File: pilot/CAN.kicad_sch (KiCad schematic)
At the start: 13 parts, among them IC1 TJA1050T, J4 Conn_01x02, U5 MCP2515-xSO, Y2 ABLS-8.000MHZ-12-B-4-Y-T

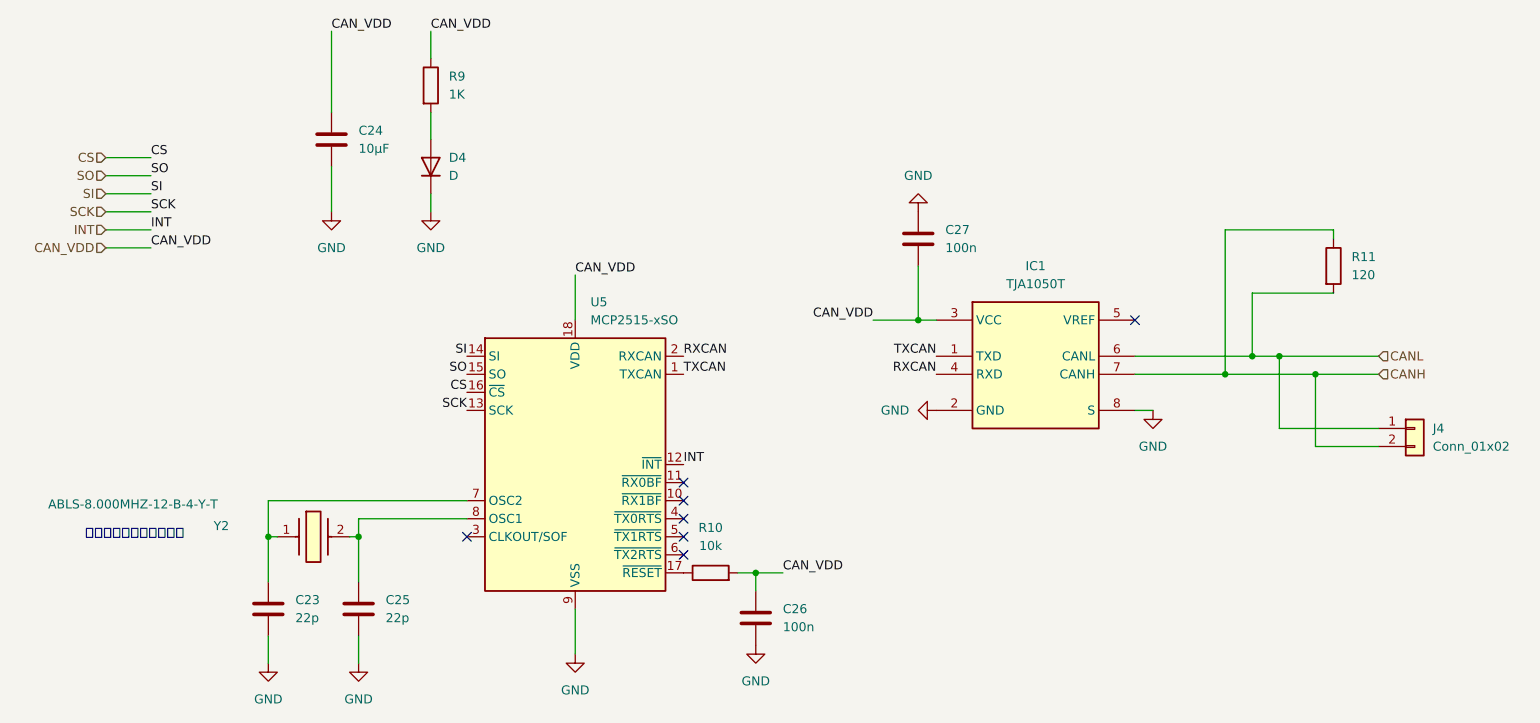
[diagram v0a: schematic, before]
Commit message: 2026/02/12/1628
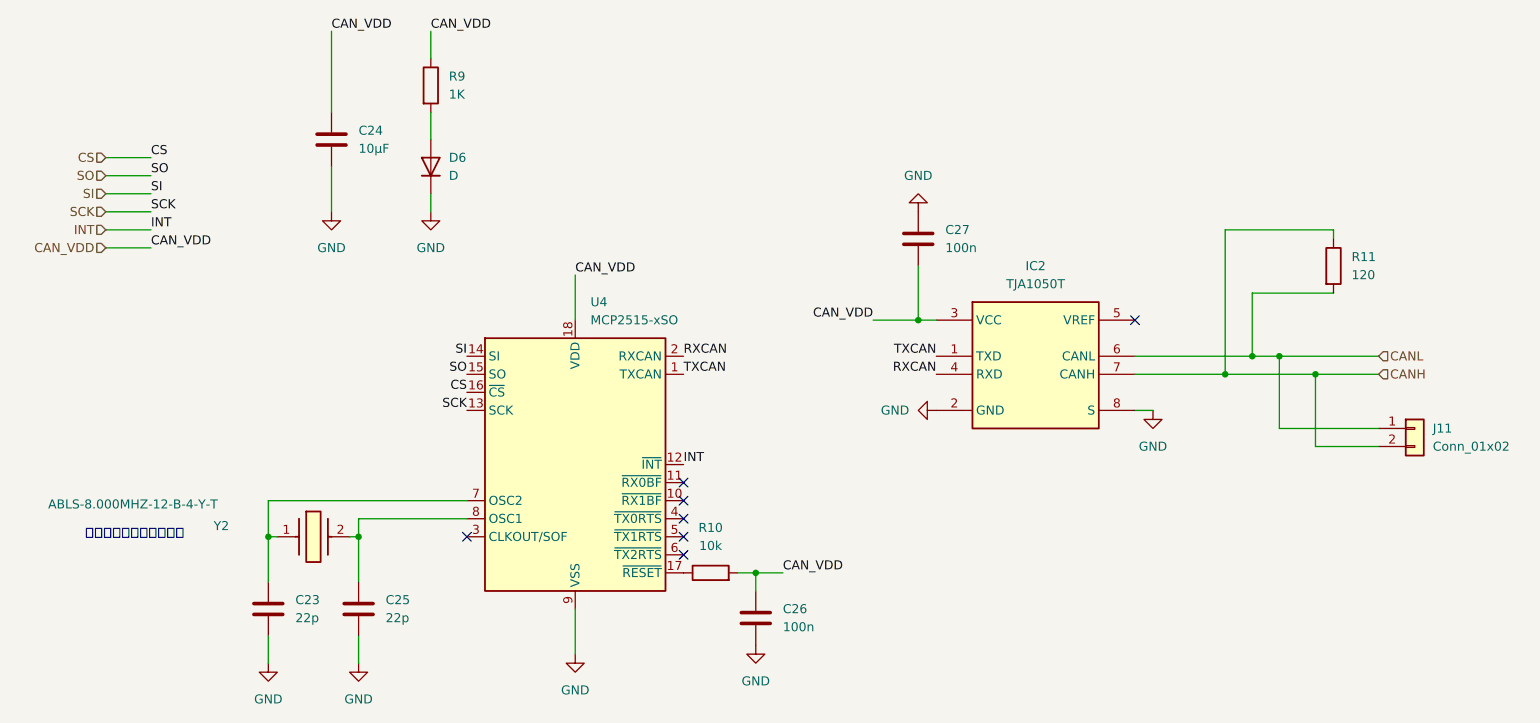
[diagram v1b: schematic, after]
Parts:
- C23, C25, C26, C27: footprint (none) -> Capacitor_SMD:C_0603_1608Metric
- C24: footprint (none) -> Capacitor_SMD:C_0805_2012Metric
- D6: renamed from D4; footprint (none) -> Diode_SMD:D_SMA
- IC2: renamed from IC1; footprint SOIC127P600X175-8N -> rp2350:SOIC127P600X175-8N
- J11: renamed from J4; footprint (none) -> Connector_PinHeader_2.54mm:PinHeader_1x02_P2.54mm_Vertical
- R10, R11, R9: footprint (none) -> Resistor_SMD:R_0603_1608Metric
- renumbered U5 to U4
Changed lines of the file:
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@@
 		(dnp no)
 		(fields_autoplaced yes)
-		(property "Reference" "#PWR044"
+		(property "Reference" "#PWR060"
 			(at 213.36 85.09 0)
 			(effects
@@
 			(project ""
 				(path "/6e01a02a-937c-45ab-a43c-49a8d1056ac9/dfd1c32f-bd86-4594-b3e8-9cea7250640c"
-					(reference "#PWR044")
+					(reference "#PWR060")
 					(unit 1)
 				)
@@
 		(dnp no)
 		(fields_autoplaced yes)
-		(property "Reference" "#PWR041"
+		(property "Reference" "#PWR057"
 			(at 157.48 118.11 0)
 			(effects
@@
 			(project ""
 				(path "/6e01a02a-937c-45ab-a43c-49a8d1056ac9/dfd1c32f-bd86-4594-b3e8-9cea7250640c"
-					(reference "#PWR041")
+					(reference "#PWR057")
 					(unit 1)
 				)
@@
 			)
 		)
-		(property "Footprint" ""
+		(property "Footprint" "Resistor_SMD:R_0603_1608Metric"
 			(at 236.982 58.42 90)
 			(effects
@@
 			)
 		)
-		(property "Footprint" ""
+		(property "Footprint" "Resistor_SMD:R_0603_1608Metric"
 			(at 109.982 33.02 90)
 			(effects
@@
 			)
 		)
-		(property "Footprint" ""
+		(property "Footprint" "Capacitor_SMD:C_0603_1608Metric"
 			(at 102.5652 110.49 0)
 			(effects
@@
 		(dnp no)
 		(fields_autoplaced yes)
-		(property "Reference" "#PWR043"
+		(property "Reference" "#PWR059"
 			(at 176.53 78.74 0)
 			(effects
@@
 			(project ""
 				(path "/6e01a02a-937c-45ab-a43c-49a8d1056ac9/dfd1c32f-bd86-4594-b3e8-9cea7250640c"
-					(reference "#PWR043")
+					(reference "#PWR059")
 					(unit 1)
 				)
@@
 			)
 		)
-		(property "Footprint" ""
+		(property "Footprint" "Capacitor_SMD:C_0805_2012Metric"
 			(at 98.7552 44.45 0)
 			(effects
@@
 			)
 		)
-		(property "Footprint" ""
+		(property "Footprint" "Capacitor_SMD:C_0603_1608Metric"
 			(at 181.3052 58.42 0)
 			(effects
@@
 		(dnp no)
 		(fields_autoplaced yes)
-		(property "Reference" "#PWR039"
+		(property "Reference" "#PWR055"
 			(at 111.76 57.15 0)
 			(effects
@@
 			(project ""
 				(path "/6e01a02a-937c-45ab-a43c-49a8d1056ac9/dfd1c32f-bd86-4594-b3e8-9cea7250640c"
-					(reference "#PWR039")
+					(reference "#PWR055")
 					(unit 1)
 				)
@@
 			)
 		)
-		(property "Footprint" ""
+		(property "Footprint" "Capacitor_SMD:C_0603_1608Metric"
 			(at 89.8652 110.49 0)
 			(effects
@@
 		(dnp no)
 		(fields_autoplaced yes)
-		(property "Reference" "#PWR037"
+		(property "Reference" "#PWR053"
 			(at 97.79 57.15 0)
 			(effects
@@
 			(project "pilot"
 				(path "/6e01a02a-937c-45ab-a43c-49a8d1056ac9/dfd1c32f-bd86-4594-b3e8-9cea7250640c"
-					(reference "#PWR037")
+					(reference "#PWR053")
 					(unit 1)
 				)
@@
 		(dnp no)
 		(fields_autoplaced yes)
-		(property "Reference" "D4"
+		(property "Reference" "D6"
 			(at 114.3 43.1799 90)
 			(effects
@@
 			)
 		)
-		(property "Footprint" ""
+		(property "Footprint" "Diode_SMD:D_SMA"
 			(at 111.76 44.45 0)
 			(effects
@@
 			(project ""
 				(path "/6e01a02a-937c-45ab-a43c-49a8d1056ac9/dfd1c32f-bd86-4594-b3e8-9cea7250640c"
-					(reference "D4")
+					(reference "D6")
 					(unit 1)
 				)
@@
 		(dnp no)
 		(fields_autoplaced yes)
-		(property "Reference" "#PWR038"
+		(property "Reference" "#PWR054"
 			(at 101.6 120.65 0)
 			(effects
@@
 			(project ""
 				(path "/6e01a02a-937c-45ab-a43c-49a8d1056ac9/dfd1c32f-bd86-4594-b3e8-9cea7250640c"
-					(reference "#PWR038")
+					(reference "#PWR054")
 					(unit 1)
 				)
@@
 			)
 		)
-		(property "Footprint" ""
+		(property "Footprint" "Resistor_SMD:R_0603_1608Metric"
 			(at 151.13 103.378 90)
 			(effects
@@
 		(dnp no)
 		(fields_autoplaced yes)
-		(property "Reference" "U5"
+		(property "Reference" "U4"
 			(at 134.2233 63.5 0)
 			(effects
@@
 			(project ""
 				(path "/6e01a02a-937c-45ab-a43c-49a8d1056ac9/dfd1c32f-bd86-4594-b3e8-9cea7250640c"
-					(reference "U5")
+					(reference "U4")
 					(unit 1)
 				)
@@
 		(on_board yes)
 		(dnp no)
-		(property "Reference" "#PWR042"
+		(property "Reference" "#PWR058"
 			(at 180.34 44.45 0)
 			(effects
@@
 			(project ""
 				(path "/6e01a02a-937c-45ab-a43c-49a8d1056ac9/dfd1c32f-bd86-4594-b3e8-9cea7250640c"
-					(reference "#PWR042")
+					(reference "#PWR058")
 					(unit 1)
 				)
@@
 		(dnp no)
 		(fields_autoplaced yes)
-		(property "Reference" "J4"
+		(property "Reference" "J11"
 			(at 252.73 81.2799 0)
 			(effects
@@
 			)
 		)
-		(property "Footprint" ""
+		(property "Footprint" "Connector_PinHeader_2.54mm:PinHeader_1x02_P2.54mm_Vertical"
 			(at 250.19 81.28 0)
 			(effects
@@
 			(project "pilot"
 				(path "/6e01a02a-937c-45ab-a43c-49a8d1056ac9/dfd1c32f-bd86-4594-b3e8-9cea7250640c"
-					(reference "J4")
+					(reference "J11")
 					(unit 1)
 				)
@@
 			)
 		)
-		(property "Footprint" ""
+		(property "Footprint" "Capacitor_SMD:C_0603_1608Metric"
 			(at 158.4452 111.76 0)
 			(effects
@@
 		(dnp no)
 		(fields_autoplaced yes)
-		(property "Reference" "#PWR036"
+		(property "Reference" "#PWR052"
 			(at 88.9 120.65 0)
 			(effects
@@
 			(project ""
 				(path "/6e01a02a-937c-45ab-a43c-49a8d1056ac9/dfd1c32f-bd86-4594-b3e8-9cea7250640c"
-					(reference "#PWR036")
+					(reference "#PWR052")
 					(unit 1)
 				)
@@
 		(dnp no)
 		(fields_autoplaced yes)
-		(property "Reference" "IC1"
+		(property "Reference" "IC2"
 			(at 196.85 58.42 0)
 			(effects
@@
 			)
 		)
-		(property "Footprint" "SOIC127P600X175-8N"
+		(property "Footprint" "rp2350:SOIC127P600X175-8N"
 			(at 207.01 160.96 0)
 			(effects
@@
 			(project ""
 				(path "/6e01a02a-937c-45ab-a43c-49a8d1056ac9/dfd1c32f-bd86-4594-b3e8-9cea7250640c"
-					(reference "IC1")
+					(reference "IC2")
 					(unit 1)
 				)
@@
 		(dnp no)
 		(fields_autoplaced yes)
-		(property "Reference" "#PWR040"
+		(property "Reference" "#PWR056"
 			(at 132.08 119.38 0)
 			(effects
@@
 			(project ""
 				(path "/6e01a02a-937c-45ab-a43c-49a8d1056ac9/dfd1c32f-bd86-4594-b3e8-9cea7250640c"
-					(reference "#PWR040")
-					(unit 1)
-				)
+					(reference "#PWR056")
+					(unit 1)
+				)
